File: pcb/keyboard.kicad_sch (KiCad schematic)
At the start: 19 parts, among them U1 Arduino_Pro_Micro

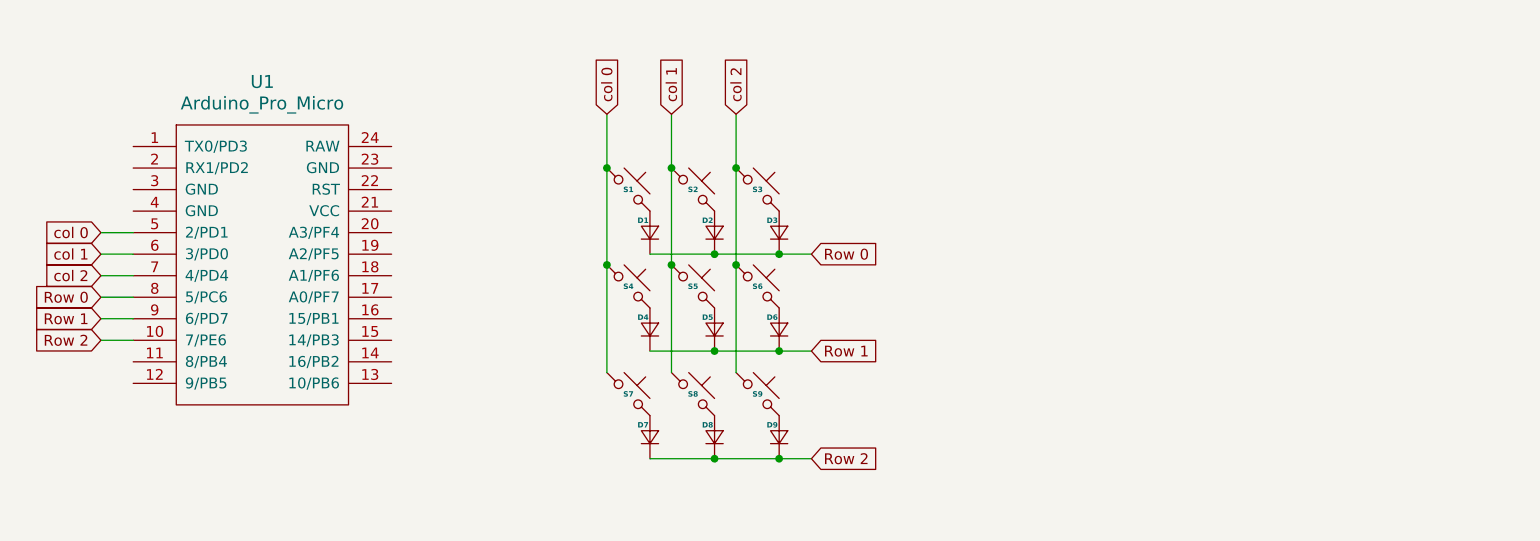
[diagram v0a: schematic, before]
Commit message: oled screen a dial new case new pc
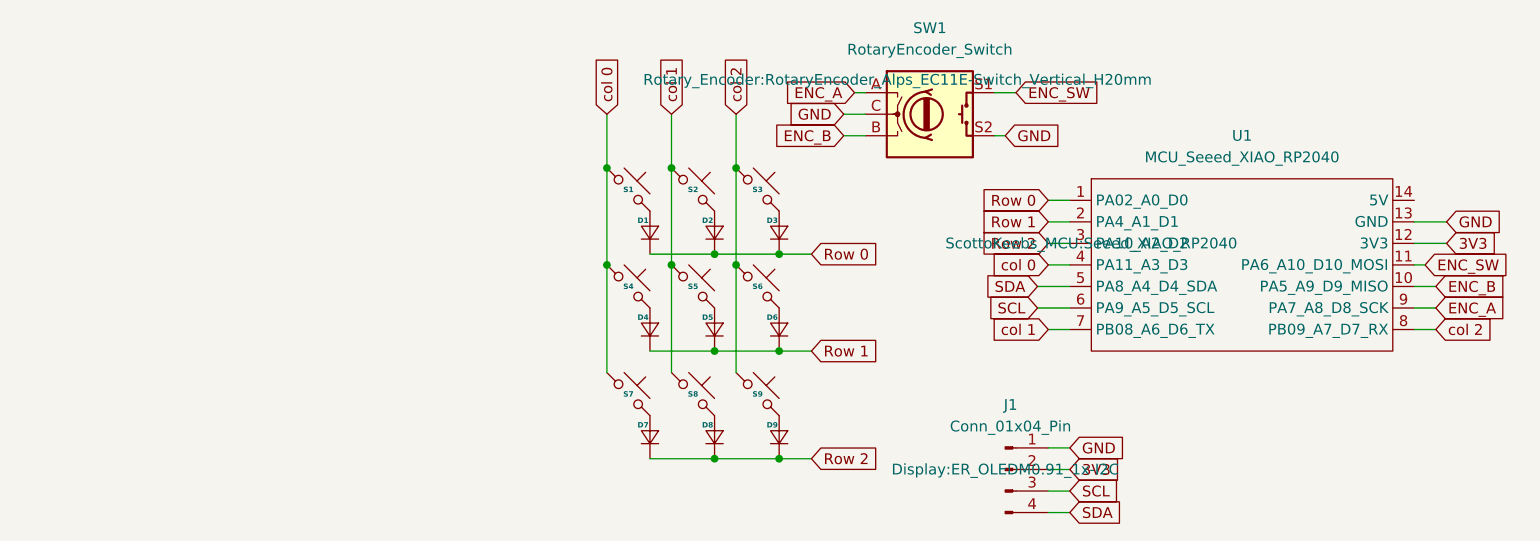
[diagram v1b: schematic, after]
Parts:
- removed U1: Arduino_Pro_Micro, ScottoKeebs_MCU:Arduino_Pro_Micro, symbol ScottoKeebs:MCU_Arduino_Pro_Micro
- added J1: Conn_01x04_Pin, Display:ER_OLEDM0.91_1x-I2C, symbol Connector:Conn_01x04_Pin
- added SW1: RotaryEncoder_Switch, Rotary_Encoder:RotaryEncoder_Alps_EC11E-Switch_Vertical_H20mm, symbol Device:RotaryEncoder_Switch
- added U1: MCU_Seeed_XIAO_RP2040, ScottoKeebs_MCU:Seeed_XIAO_RP2040, symbol ScottoKeebs:MCU_Seeed_XIAO_RP2040
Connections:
- net Row 0: now also U1.1 (PA02_A0_D0)
- net Row 1: now also U1.2 (PA4_A1_D1)
- net Row 2: now also U1.3 (PA10_A2_D2)
- net col 0: now also U1.4 (PA11_A3_D3)
- net col 1: now also U1.7 (PB08_A6_D6_TX)
- net col 2: now also U1.8 (PB09_A7_D7_RX)
- new net 3V3: J1.2 (Pin_2), U1.12 (3V3)
- new net ENC_A: SW1.A, U1.9 (PA7_A8_D8_SCK)
- new net ENC_B: SW1.B, U1.10 (PA5_A9_D9_MISO)
- new net ENC_SW: SW1.S1, U1.11 (PA6_A10_D10_MOSI)
- new net GND: J1.1 (Pin_1), SW1.C, SW1.S2, U1.13 (GND)
- new net SCL: J1.3 (Pin_3), U1.6 (PA9_A5_D5_SCL)
- new net SDA: J1.4 (Pin_4), U1.5 (PA8_A4_D4_SDA)
